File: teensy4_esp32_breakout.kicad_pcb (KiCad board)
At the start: 2 copper layers, 30.5 x 22.9 mm, 16 parts, among them J1 Conn_01x08, J2 Conn_02x05_Odd_Even, SW1 ON_OFF, U1 ESP32-WROOM-32D, U2 TLV75533PDBV

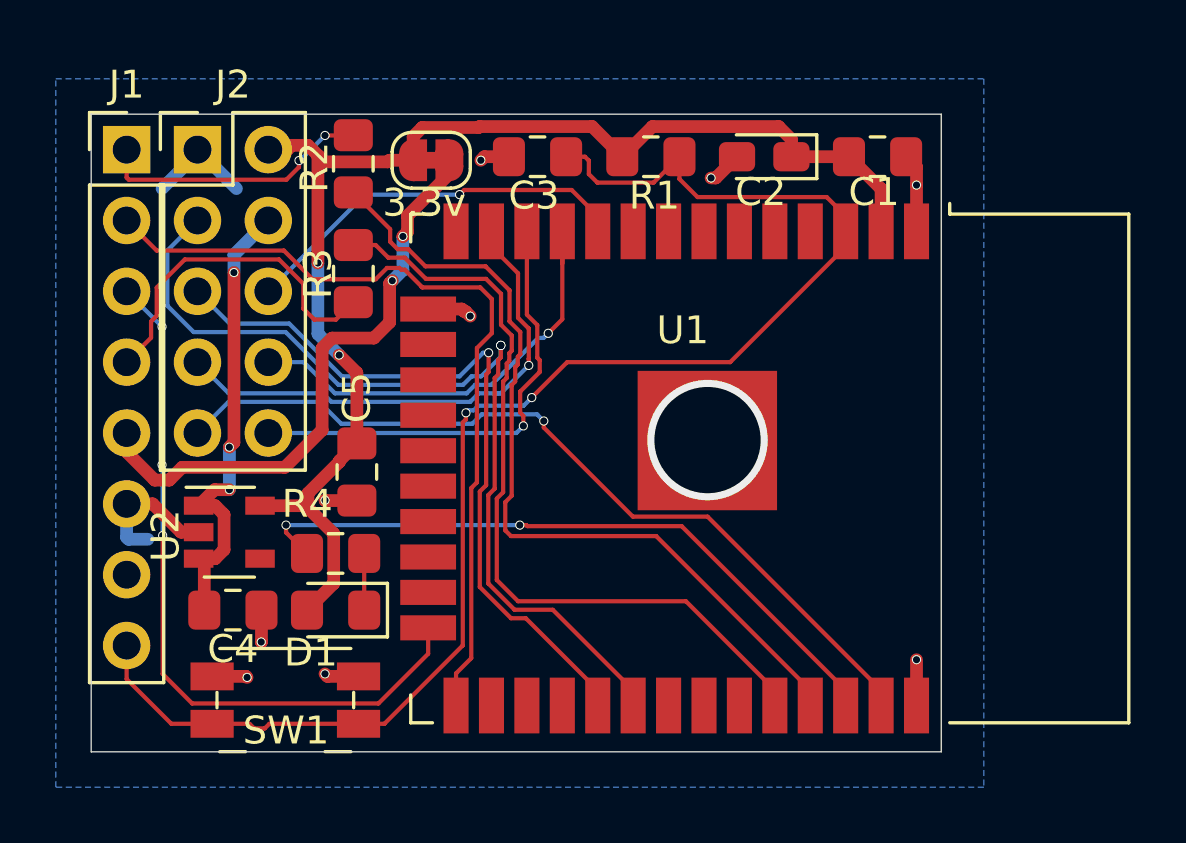
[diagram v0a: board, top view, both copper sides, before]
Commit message: Forgot to save
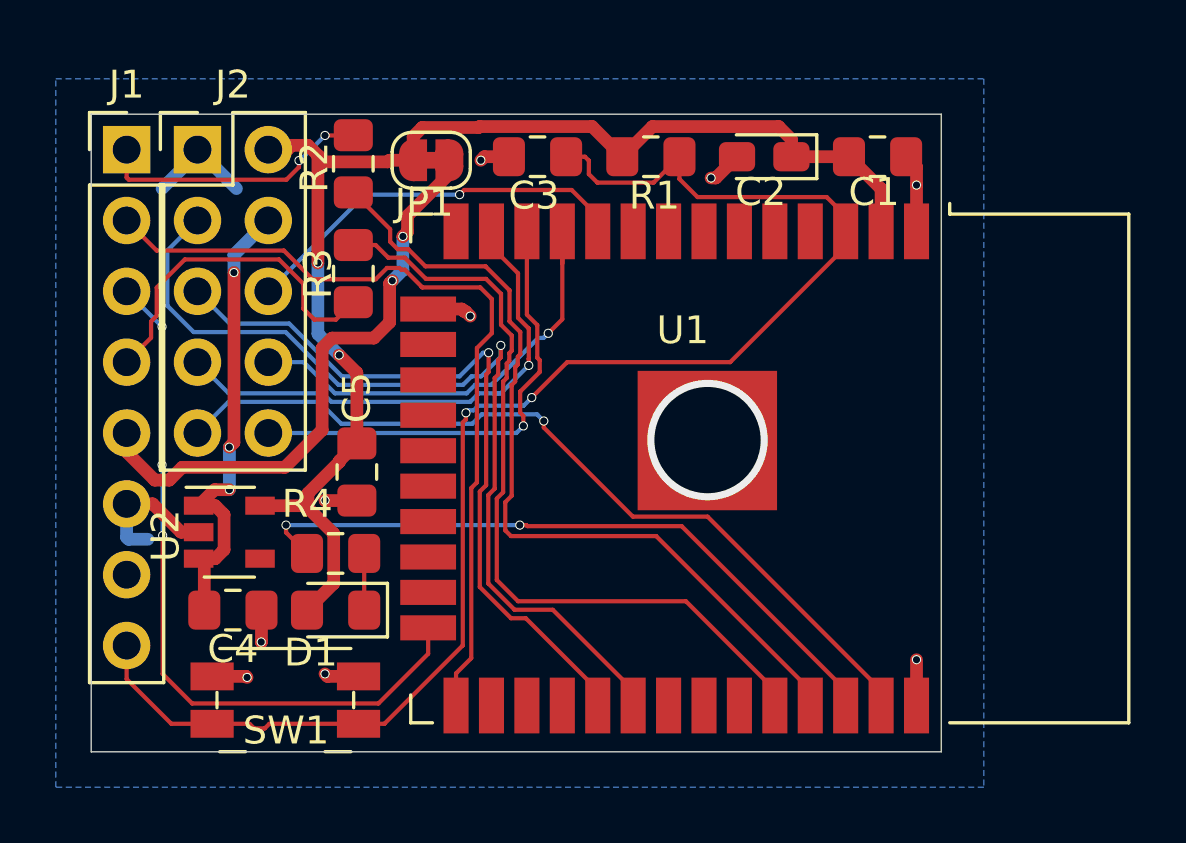
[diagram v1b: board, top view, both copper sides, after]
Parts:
- renumbered 3.3v to JP1
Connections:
- U1 pad 39: GND -> (no net)
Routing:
- net GND: vias 10 -> 9
- net /SCK: vias 2 -> 1
- net (no net): vias 0 -> 1
